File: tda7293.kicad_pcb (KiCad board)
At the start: 2 copper layers, 100 x 60 mm, 76 parts, among them J1 Screw_Terminal_01x04, J2 Conn_01x01_Male, J3 Screw_Terminal_01x02, J4 Conn_01x01_Male, J5 Conn_01x01_Male, J6 Conn_01x01_Male, J7 Conn_01x01_Male, J8 Conn_01x01_Male, J9 Conn_01x01_Male, Q1 BSS84, Q2 2N7002, U1 TDA7293, U2 TDA7293, U3 PC817, U4 MCP1792

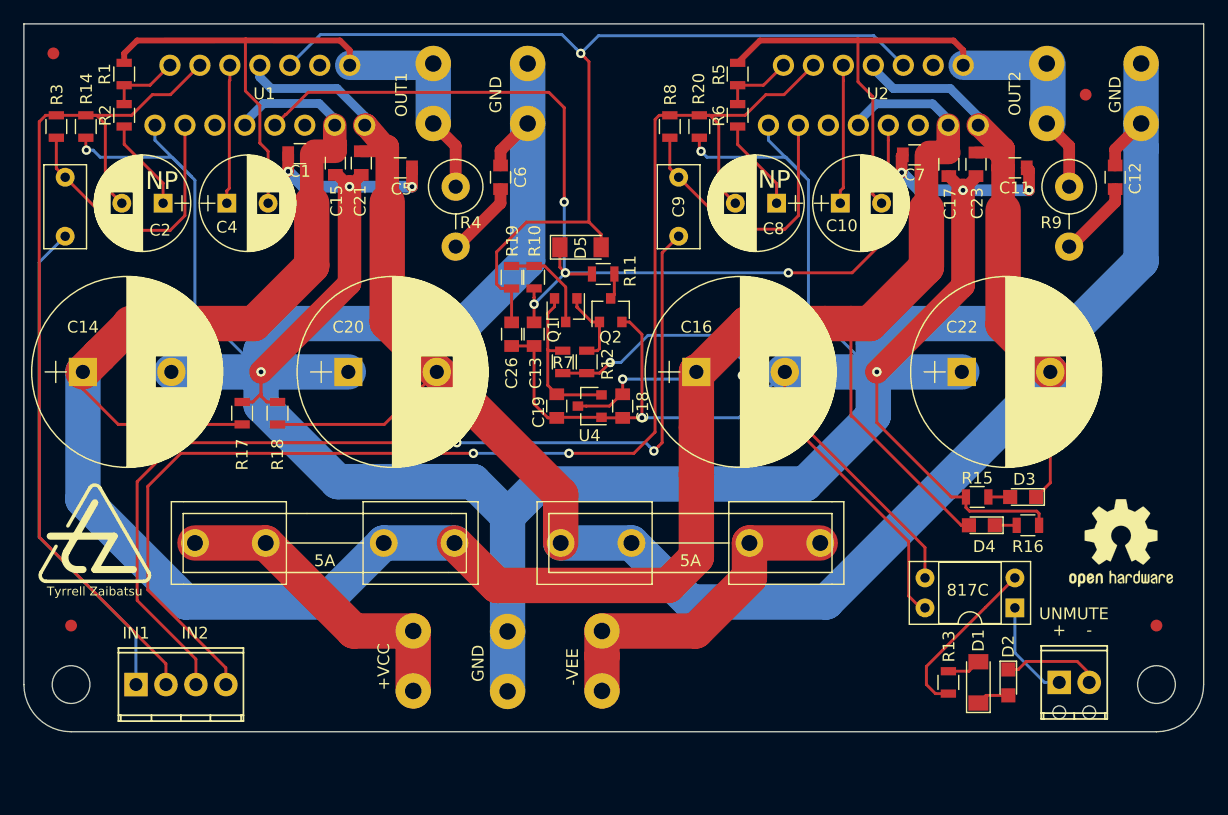
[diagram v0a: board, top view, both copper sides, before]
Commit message: silk-screen updates, turd-polishing, plotted gerbers
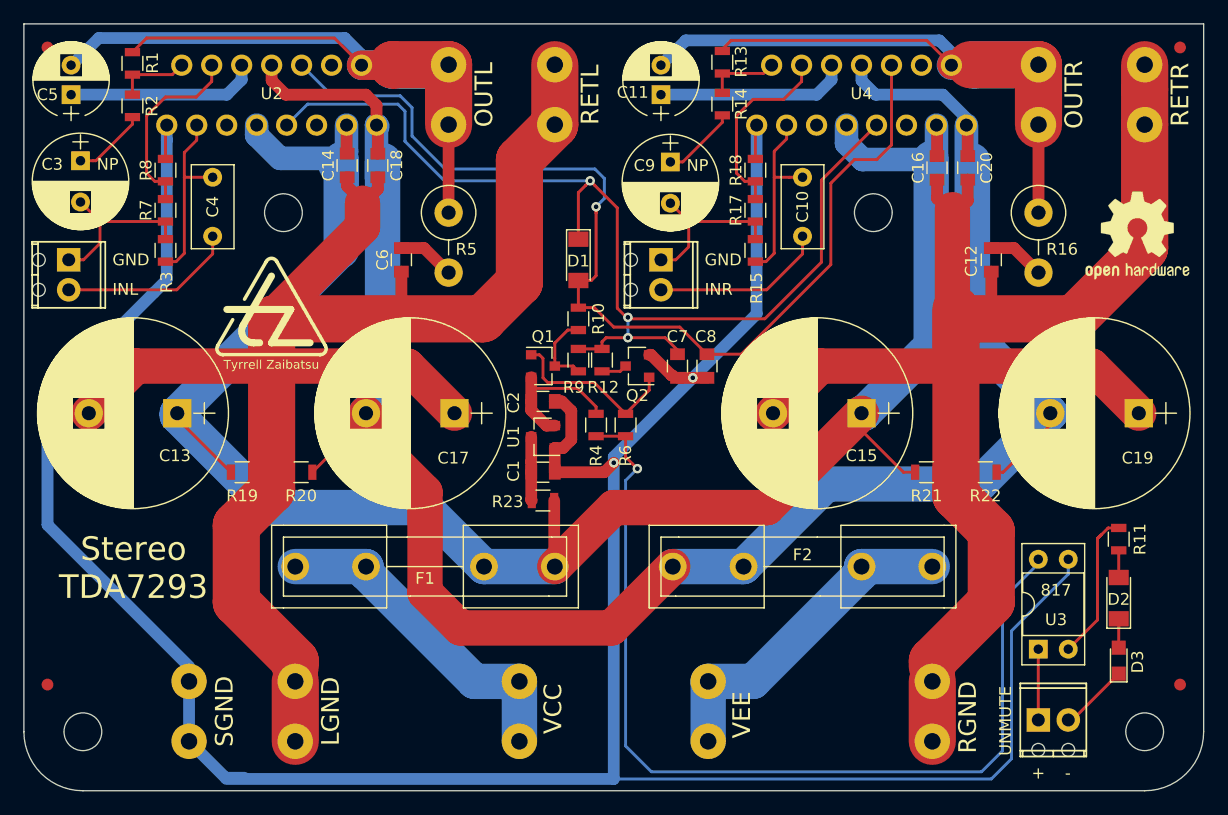
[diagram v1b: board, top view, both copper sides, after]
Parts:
- removed C21, C23: 1u, Capacitors_SMD:C_0805
- removed C22: 1000u, Capacitors_ThroughHole:CP_Radial_D16.0mm_P7.50mm
- removed C26: 10u, Capacitors_SMD:C_0805
- removed D4: LED, LEDs:LED_0805
- removed D5: LL4148, Diodes_SMD:D_MiniMELF
- removed the REF*** at (106.0, 62.0)
- added H3: MountingHole, Mounting_Holes:MountingHole_3.2mm_M3, F.Cu at (47.0, 41.0)
- added H4: MountingHole, Mounting_Holes:MountingHole_3.2mm_M3, F.Cu at (97.0, 41.0)
- added J10: Conn_01x01_Male, power:FASTON250P_5.08mm_male_vertical, F.Cu at (48.0, 83.3)
- added J11: Conn_01x01_Male, power:FASTON250P_5.08mm_male_vertical, F.Cu at (102.0, 83.3)
- added J12: Conn_01x01_Male, power:FASTON250P_5.08mm_male_vertical, F.Cu at (83.0, 83.3)
- added R21: 27k, Resistors_SMD:R_0805, F.Cu at (101.5, 63.0)
- added R22: 27k, Resistors_SMD:R_0805, F.Cu at (106.5, 63.0)
- added R23: 1k, Resistors_SMD:R_0805, F.Cu at (69.0, 65.4)
- C10, C4: value 22u -> 1u; footprint Capacitors_ThroughHole:CP_Radial_D8.0mm_P3.50mm -> Capacitors_ThroughHole:C_Rect_L7.0mm_W3.5mm_P5.00mm
- C11, C5: value 1u -> 22u; footprint Capacitors_SMD:C_0805 -> Capacitors_ThroughHole:CP_Radial_D6.3mm_P2.50mm
- C13, C19: value 10u -> 1000u; footprint Capacitors_SMD:C_0805 -> Capacitors_ThroughHole:CP_Radial_D16.0mm_P7.50mm
- C14, C16, C20: value 1000u -> 1u; footprint Capacitors_ThroughHole:CP_Radial_D16.0mm_P7.50mm -> Capacitors_SMD:C_0805
- C15, C17: value 1u -> 1000u; footprint Capacitors_SMD:C_0805 -> Capacitors_ThroughHole:CP_Radial_D16.0mm_P7.50mm
- C2, C8: value 22u NP -> 10u; footprint Capacitors_ThroughHole:CP_Radial_D8.0mm_P3.50mm -> Capacitors_SMD:C_0805
- C3, C9: value 1u -> 22u NP; footprint Capacitors_ThroughHole:C_Rect_L7.0mm_W3.5mm_P5.00mm -> Capacitors_ThroughHole:CP_Radial_D8.0mm_P3.50mm
- C7: value 1u -> 10u
- D2: value LED -> LL4148; footprint LEDs:LED_0805 -> Diodes_SMD:D_MiniMELF
- J1: value Screw_Terminal_01x04 -> Screw_Terminal_01x02; footprint Terminals_Phoenix:TerminalBlock_Phoenix_MPT-2.54mm_4pol -> Terminals_Phoenix:TerminalBlock_Phoenix_MPT-2.54mm_2pol
- J6: value Conn_01x01_Male -> Screw_Terminal_01x02; footprint power:FASTON250P_5.08mm_male_vertical -> Terminals_Phoenix:TerminalBlock_Phoenix_MPT-2.54mm_2pol
- R10: value 10k -> 27k
- R11: value 1k -> 3k9
- R12: value 100 -> 1k
- R13: value 3k9 -> 22k
- R14: value 15 -> 680
- R15: value 10k -> 22k
- R16: value 10k -> 2R7; footprint Resistors_SMD:R_0805 -> Resistors_ThroughHole:R_Axial_DIN0414_L11.9mm_D4.5mm_P5.08mm_Vertical
- R17: value 27k -> 10
- R18: value 27k -> 0R
- R20: value 15 -> 27k
- R4, R9: value 2R7 -> 10k; footprint Resistors_ThroughHole:R_Axial_DIN0414_L11.9mm_D4.5mm_P5.08mm_Vertical -> Resistors_SMD:R_0805
- R5: value 22k -> 2R7; footprint Resistors_SMD:R_0805 -> Resistors_ThroughHole:R_Axial_DIN0414_L11.9mm_D4.5mm_P5.08mm_Vertical
- R6: value 680 -> 100
- R7: value 10k -> 10
- R8: value 22k -> 0R
- U1: value TDA7293 -> MCP1792; footprint power:Multiwatt15V -> TO_SOT_Packages_SMD:SOT-23
- U4: value MCP1792 -> TDA7293; footprint TO_SOT_Packages_SMD:SOT-23 -> power:Multiwatt15V
- moved FID1 106.0 mm to (27.0, 27.0)
- moved FID4 94.1 mm to (123.0, 81.0)
- moved J5 89.6 mm to (39.0, 83.3)
- moved J8 72.3 mm to (120.0, 31.0), turned to 0 degrees
- moved J7 71.5 mm to (111.0, 31.0)
- moved R13 56.0 mm to (84.2, 28.2), turned to 90 degrees
- moved C20 55.3 mm to (105.0, 37.2), turned to 90 degrees
- moved R14 54.0 mm to (84.2, 31.8)
- moved FID3 53.5 mm to (27.0, 81.0)
- moved U2 51.0 mm to (46.0, 28.5)
- moved C15 49.4 mm to (96.0, 58.0), turned to 180 degrees
- moved C19 49.3 mm to (119.5, 58.0), turned to 180 degrees
- moved D1 49.3 mm to (72.0, 45.0), turned to 270 degrees
- moved R11 49.1 mm to (117.8, 68.7), turned to 90 degrees
- moved C17 46.9 mm to (61.5, 58.0), turned to 180 degrees
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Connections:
- C1 pad 1: /VCC -> Net-(C1-Pad1)
- C1 pad 2: /GND -> /SGND
- C10 pad 2: /OUT2 -> Net-(C10-Pad2)
- C11 pad 1: /GND -> Net-(C11-Pad1)
- C11 pad 2: /VEE -> /OUTR
- C12 pad 2: /GND -> /RGND
- C13 pad 1: /GND -> /VCC
- C13 pad 2: /STBY -> /LGND
- C14 pad 2: /GND -> /LGND
- C15 pad 2: /GND -> /RGND
- C16 pad 2: /GND -> /RGND
- C17 pad 1: /VCC -> /LGND
- C17 pad 2: /GND -> /VEE
- C18 pad 1: /VCC -> /LGND
- C18 pad 2: /GND -> /VEE
- C19 pad 1: /5V -> /RGND
- C19 pad 2: /GND -> /VEE
- C2 pad 1: Net-(C2-Pad1) -> /5V
- C2 pad 2: Net-(C2-Pad2) -> /SGND
- C20 pad 1: /GND -> /RGND
- C4 pad 2: /OUT1 -> Net-(C4-Pad2)
- C5 pad 1: /GND -> Net-(C5-Pad1)
- C5 pad 2: /VEE -> /OUTL
- C6 pad 2: /GND -> /LGND
- C7 pad 1: /VCC -> /SGND
- C7 pad 2: /GND -> /STBY
- C8 pad 1: Net-(C8-Pad1) -> /SGND
- C8 pad 2: Net-(C8-Pad2) -> /MUTE
- D1 pad 1: Net-(D1-Pad1) -> /STBY
- D1 pad 2: Net-(D1-Pad2) -> /MUTE
- D2 pad 2: Net-(D1-Pad1) -> Net-(D2-Pad2)
- D3 pad 1: /VEE -> Net-(D3-Pad1)
- D3 pad 2: Net-(D3-Pad2) -> Net-(D2-Pad1)
- J1 pad 2: Net-(C2-Pad2) -> Net-(C4-Pad2)
- J2 pad 1: /OUT1 -> /OUTL
- J3 pad 2: Net-(D2-Pad1) -> Net-(D3-Pad1)
- J4 pad 1: /GND -> /LGND
- J5 pad 1: /OUT2 -> /SGND
- J6 pad 1: /GND -> Net-(C9-Pad2)
- J7 pad 1: Net-(F1-Pad2) -> /OUTR
- J8 pad 1: /GND -> /RGND
- J9 pad 1: Net-(F2-Pad2) -> Net-(F1-Pad2)
- Q2 pad 2: /GND -> /SGND
- R1 pad 2: /OUT1 -> /OUTL
- R10 pad 2: /STBY -> /MUTE
- R11 pad 1: /STBY -> Net-(D2-Pad2)
- R11 pad 2: Net-(Q2-Pad3) -> Net-(R11-Pad2)
- R12 pad 1: Net-(R12-Pad1) -> /STBY
- R12 pad 2: Net-(Q1-Pad1) -> Net-(Q2-Pad3)
- R13 pad 1: Net-(D1-Pad2) -> Net-(R13-Pad1)
- R13 pad 2: Net-(R13-Pad2) -> /OUTR
- R14 pad 1: Net-(C2-Pad2) -> Net-(R13-Pad1)
- R14 pad 2: /GND -> Net-(C9-Pad1)
- R15 pad 1: /GND -> Net-(C9-Pad2)
- R15 pad 2: Net-(D3-Pad2) -> Net-(C10-Pad1)
- R16 pad 1: Net-(D4-Pad1) -> /OUTR
- R16 pad 2: /GND -> Net-(C12-Pad1)
- R17 pad 1: /GND -> Net-(C9-Pad2)
- R17 pad 2: /VCC -> Net-(R17-Pad2)
- R18 pad 1: /VEE -> Net-(R17-Pad2)
- R18 pad 2: /GND -> /SGND
- R19 pad 1: Net-(Q1-Pad3) -> /LGND
- R19 pad 2: /MUTE -> /VCC
- R2 pad 2: Net-(C2-Pad1) -> Net-(C3-Pad1)
- R20 pad 1: Net-(C8-Pad2) -> /VEE
- R20 pad 2: /GND -> /LGND
- R3 pad 1: Net-(C2-Pad2) -> Net-(C3-Pad2)
- R3 pad 2: Net-(C3-Pad1) -> Net-(C4-Pad1)
- R4 pad 1: /OUT1 -> Net-(R4-Pad1)
- R4 pad 2: Net-(C6-Pad1) -> /5V
- R5 pad 1: Net-(R5-Pad1) -> /OUTL
- R5 pad 2: /OUT2 -> Net-(C6-Pad1)
- R6 pad 1: Net-(R5-Pad1) -> Net-(R4-Pad1)
- R6 pad 2: Net-(C8-Pad1) -> Net-(Q1-Pad1)
- R7 pad 1: Net-(R12-Pad1) -> Net-(C3-Pad2)
- R7 pad 2: /5V -> Net-(R7-Pad2)
- R8 pad 1: Net-(C8-Pad2) -> Net-(R7-Pad2)
- R8 pad 2: Net-(C9-Pad1) -> /SGND
- R9 pad 1: /OUT2 -> Net-(Q1-Pad3)
- R9 pad 2: Net-(C12-Pad1) -> /STBY
- U1 pad 1: /GND -> /SGND
- U1 pad 2: Net-(R1-Pad1) -> /5V
- U1 pad 3: Net-(C3-Pad1) -> Net-(C1-Pad1)
- U2 pad 1: /GND -> /SGND
- U2 pad 14: /OUT2 -> /OUTL
- U2 pad 2: Net-(R5-Pad1) -> Net-(R1-Pad1)
- U2 pad 3: Net-(C9-Pad1) -> Net-(C4-Pad1)
- U2 pad 4: Net-(C8-Pad2) -> Net-(R7-Pad2)
- U2 pad 5: /CLIP2 -> /CLIP1
- U2 pad 6: Net-(C10-Pad1) -> Net-(C5-Pad1)
- U3 pad 2: Net-(R13-Pad2) -> Net-(R11-Pad2)
- U3 pad 3: /GND -> /SGND
- U3 pad 4: Net-(R12-Pad1) -> Net-(R4-Pad1)
- U4 pad 1: /GND -> /SGND
- U4 pad 2: /5V -> Net-(R13-Pad1)
- U4 pad 3: /VCC -> Net-(C10-Pad1)
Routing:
- net /GND: track 442.9 -> 0.00 mm, vias 11 -> 0
- net /SGND: track 0.00 -> 239.0 mm, vias 0 -> 2
- net /LGND: track 0.00 -> 140.7 mm
- net /RGND: track 0.00 -> 127.0 mm
- net Net-(C8-Pad2): track 115.5 -> 0.00 mm, vias 2 -> 0
- net Net-(R4-Pad1): track 0.00 -> 81.3 mm, vias 0 -> 1
- net /OUTR: track 0.00 -> 77.3 mm
- net Net-(C2-Pad2): track 77.0 -> 0.00 mm
- net /OUTL: track 0.00 -> 76.9 mm
- net Net-(C9-Pad2): track 83.8 -> 14.3 mm, vias 2 -> 0
- net /VCC: track 229.9 -> 168.1 mm, vias 1 -> 0
- net /OUT1: track 55.0 -> 0.00 mm
- net /OUT2: track 54.6 -> 0.00 mm
- net Net-(R12-Pad1): track 45.1 -> 0.00 mm, vias 2 -> 0
- net Net-(C3-Pad2): track 42.3 -> 14.5 mm
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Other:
- board size 100 x 60 mm -> 100 x 65 mm
- board text added: "817"
- board text added: "INL"
- board text added: "INR"
- board text added: "LGND"
- board text added: "OUTL"
- board text added: "OUTR"
- board text added: "RETL"
- board text added: "RETR"
- board text added: "RGND"
- board text added: "SGND"
- board text added: "Stereo TDA7293"
- board text added: "Stereo TDA7293/TDA7294 Rev.B 202204 william@brodie-tyrrell.org github.com/phenidone"
- board text added: "VCC"
- board text added: "VEE"
- board text removed: "+VCC"
- board text removed: "-VEE"
- board text removed: "5A"
- board text removed: "817C"
- board text removed: "IN1"
- board text removed: "IN2"
- board text removed: "OUT1"
- board text removed: "OUT2"
- board text removed: "Stereo TDA7293/TDA7294 Rev.B 202201 william@brodie-tyrrell.org github.com/phenidone"
